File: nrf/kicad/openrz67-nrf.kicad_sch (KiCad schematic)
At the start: 15 parts, among them J1 Camera, J2 SWD, Q1 AO3401A, SW1 B3U-1000P, U1 E73-2G4M08S1F, U2 TLP172AM, U3 TLP172AM

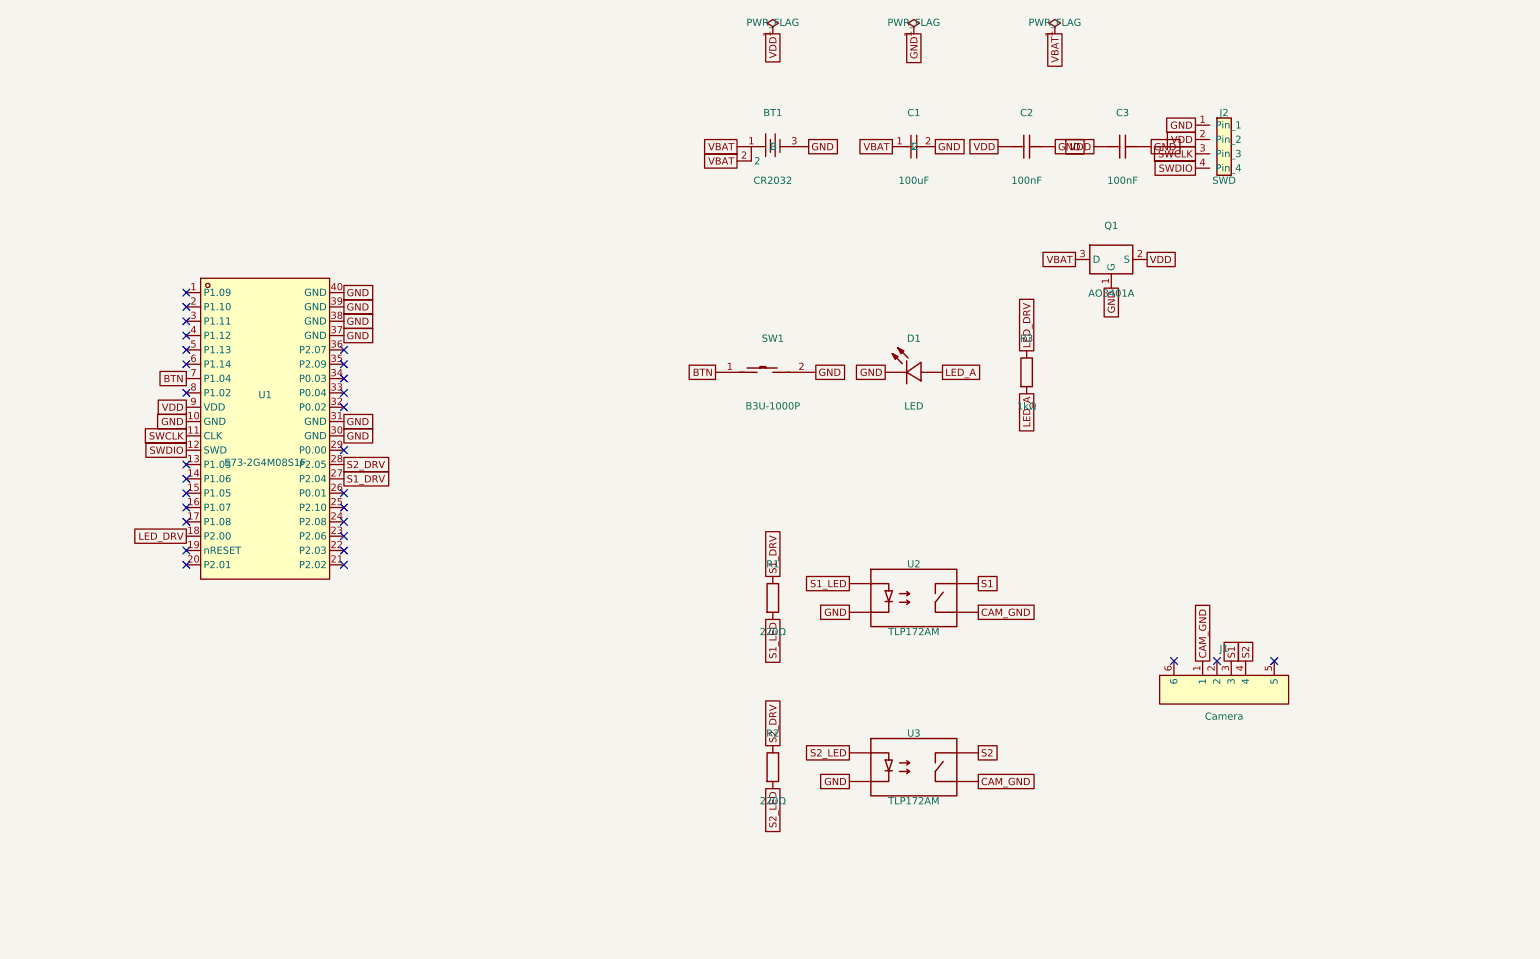
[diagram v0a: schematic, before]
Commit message: nrf: readable schematic layout
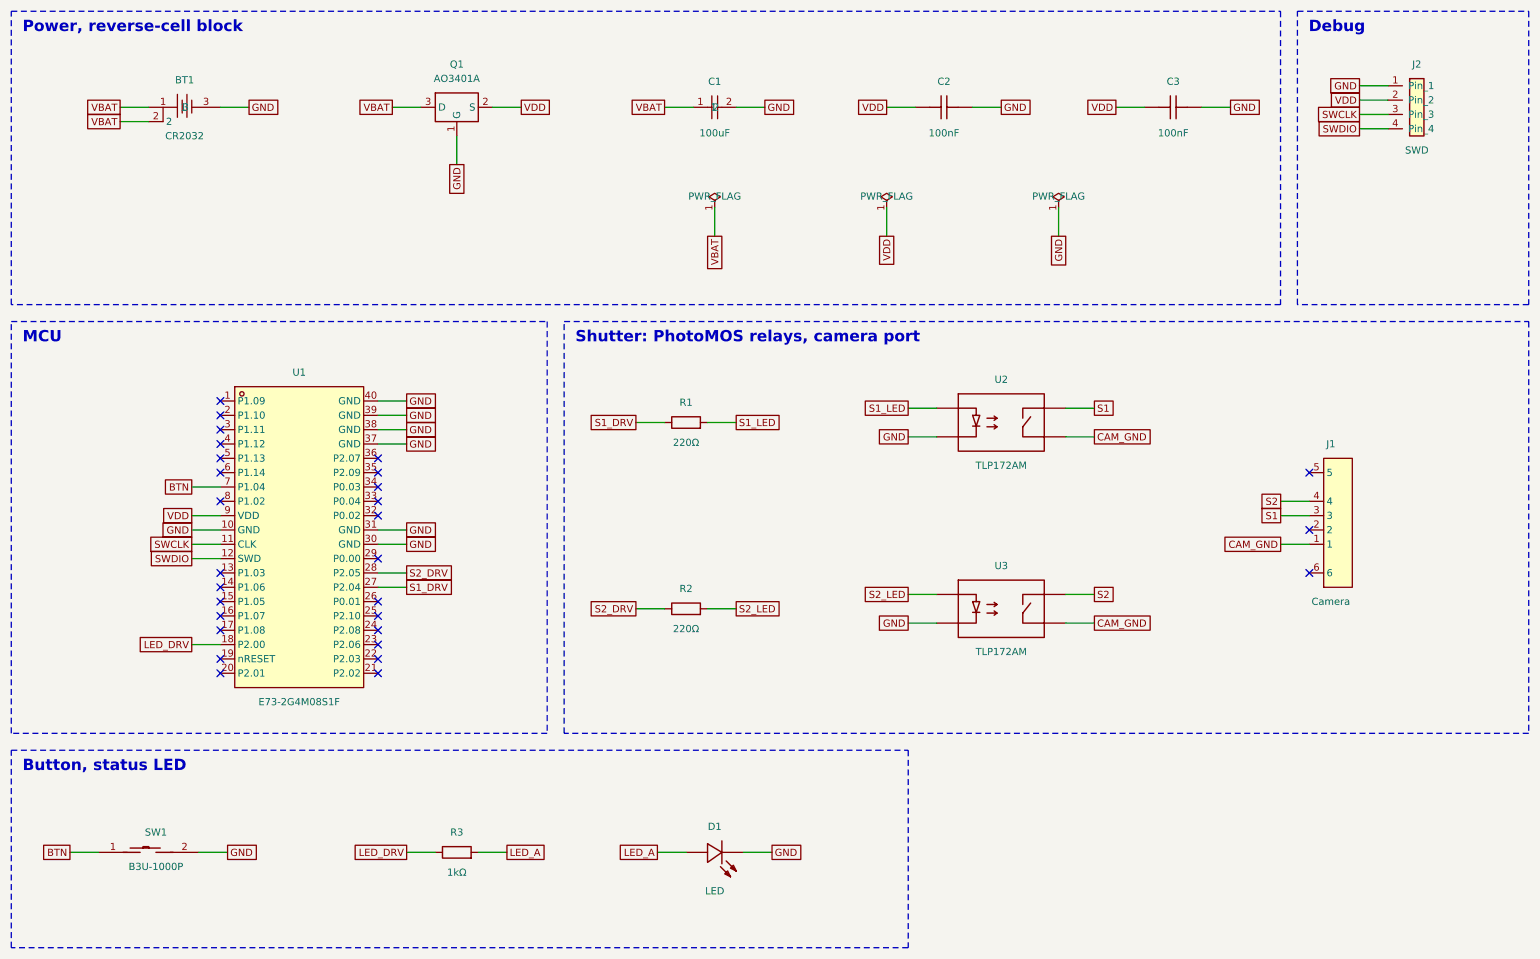
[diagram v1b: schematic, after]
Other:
- note added: "Button, status LED"
- note added: "Debug"
- note added: "MCU"
- note added: "Power, reverse-cell block"
- note added: "Shutter: PhotoMOS relays, camera port"
